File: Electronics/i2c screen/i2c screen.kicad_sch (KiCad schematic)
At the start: 4 parts, among them J1 renc_con, J2 display_con, J3 display_in, SW1 RotaryEncoder_Switch

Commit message: placement!
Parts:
- J1, J2, J3: footprint (none) -> Connector_PinHeader_2.54mm:PinHeader_1x04_P2.54mm_Vertical
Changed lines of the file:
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@@
 			)
 		)
-		(property "Footprint" ""
+		(property "Footprint" "Connector_PinHeader_2.54mm:PinHeader_1x04_P2.54mm_Vertical"
 			(at 101.6 76.2 0)
 			(effects
@@
 			)
 		)
-		(property "Footprint" ""
+		(property "Footprint" "Connector_PinHeader_2.54mm:PinHeader_1x04_P2.54mm_Vertical"
 			(at 123.19 60.96 0)
 			(effects
@@
 			)
 		)
-		(property "Footprint" ""
+		(property "Footprint" "Connector_PinHeader_2.54mm:PinHeader_1x04_P2.54mm_Vertical"
 			(at 116.84 76.2 0)
 			(effects

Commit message: updated footprints
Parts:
- J3: footprint Connector_PinHeader_2.54mm:PinHeader_1x04_P2.54mm_Vertical -> ledscreen:128x64OLED
- SW1: footprint (none) -> Rotary_Encoder:RotaryEncoder_Bourns_Vertical_PEC12R-3x17F-Sxxxx
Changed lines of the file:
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@@
 			)
 		)
-		(property "Footprint" ""
+		(property "Footprint" "Rotary_Encoder:RotaryEncoder_Bourns_Vertical_PEC12R-3x17F-Sxxxx"
 			(at 158.75 56.896 0)
 			(effects
@@
 			)
 		)
-		(property "Footprint" "Connector_PinHeader_2.54mm:PinHeader_1x04_P2.54mm_Vertical"
+		(property "Footprint" "ledscreen:128x64OLED"
 			(at 116.84 76.2 0)
 			(effects

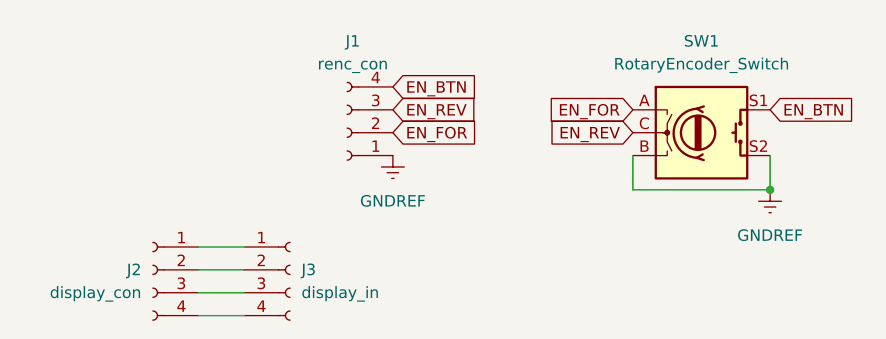
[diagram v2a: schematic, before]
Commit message: routing finito and placemnt aswell
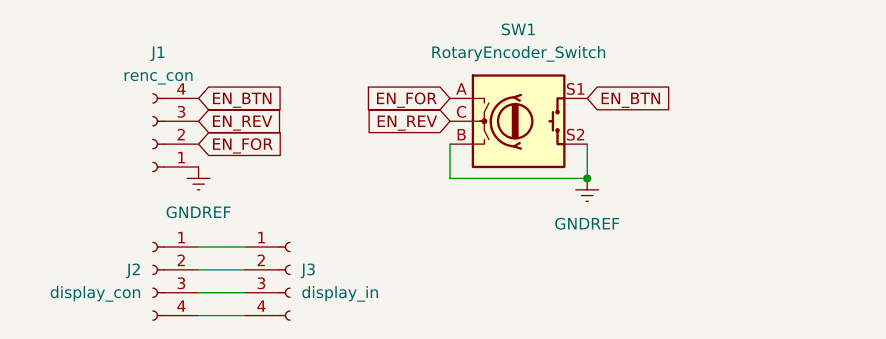
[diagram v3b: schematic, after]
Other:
- moved on the sheet: J1, SW1
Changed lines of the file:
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@@
 	(paper "A4")
 	(junction
-		(at 170.18 67.31)
+		(at 149.86 66.04)
 		(diameter 0)
 		(color 0 0 0 0)
@@
 	(wire
 		(pts
-			(xy 170.18 67.31) (xy 170.18 63.5)
+			(xy 149.86 66.04) (xy 149.86 62.23)
 		)
 		(stroke
@@
 	(wire
 		(pts
-			(xy 154.94 63.5) (xy 154.94 67.31)
+			(xy 134.62 62.23) (xy 134.62 66.04)
 		)
 		(stroke
@@
 	(wire
 		(pts
-			(xy 154.94 67.31) (xy 170.18 67.31)
+			(xy 134.62 66.04) (xy 149.86 66.04)
 		)
 		(stroke
@@
 	(global_label "EN_REV"
 		(shape input)
-		(at 154.94 60.96 180)
+		(at 134.62 59.69 180)
 		(fields_autoplaced yes)
 		(effects
@@
 		)
 		(property "Intersheetrefs" "${INTERSHEET_REFS}"
-			(at 145.0001 60.96 0)
+			(at 124.6801 59.69 0)
 			(effects
 				(font
@@
 	(global_label "EN_REV"
 		(shape input)
-		(at 128.27 58.42 0)
+		(at 106.68 59.69 0)
 		(fields_autoplaced yes)
 		(effects
@@
 		)
 		(property "Intersheetrefs" "${INTERSHEET_REFS}"
-			(at 138.2099 58.42 0)
+			(at 116.6199 59.69 0)
 			(effects
 				(font
@@
 	(global_label "EN_BTN"
 		(shape input)
-		(at 170.18 58.42 0)
+		(at 149.86 57.15 0)
 		(fields_autoplaced yes)
 		(effects
@@
 		)
 		(property "Intersheetrefs" "${INTERSHEET_REFS}"
-			(at 180.1804 58.42 0)
+			(at 159.8604 57.15 0)
 			(effects
 				(font
@@
 	(global_label "EN_FOR"
 		(shape input)
-		(at 128.27 60.96 0)
+		(at 106.68 62.23 0)
 		(fields_autoplaced yes)
 		(effects
@@
 		)
 		(property "Intersheetrefs" "${INTERSHEET_REFS}"
-			(at 138.3914 60.96 0)
+			(at 116.8014 62.23 0)
 			(effects
 				(font
@@
 	(global_label "EN_FOR"
 		(shape input)
-		(at 154.94 58.42 180)
+		(at 134.62 57.15 180)
 		(fields_autoplaced yes)
 		(effects
@@
 		)
 		(property "Intersheetrefs" "${INTERSHEET_REFS}"
-			(at 144.8186 58.42 0)
+			(at 124.4986 57.15 0)
 			(effects
 				(font
@@
 	(global_label "EN_BTN"
 		(shape input)
-		(at 128.27 55.88 0)
+		(at 106.68 57.15 0)
 		(fields_autoplaced yes)
 		(effects
@@
 		)
 		(property "Intersheetrefs" "${INTERSHEET_REFS}"
-			(at 138.2704 55.88 0)
+			(at 116.6804 57.15 0)
 			(effects
 				(font
@@
 	(symbol
 		(lib_id "Connector:Conn_01x04_Socket")
-		(at 123.19 60.96 180)
+		(at 101.6 62.23 180)
 		(unit 1)
 		(exclude_from_sim no)
@@
 		(fields_autoplaced yes)
 		(property "Reference" "J1"
-			(at 123.825 50.8 0)
+			(at 102.235 52.07 0)
 			(effects
 				(font
@@
 		)
 		(property "Value" "renc_con"
-			(at 123.825 53.34 0)
+			(at 102.235 54.61 0)
 			(effects
 				(font
@@
 		)
 		(property "Footprint" "Connector_PinHeader_2.54mm:PinHeader_1x04_P2.54mm_Vertical"
-			(at 123.19 60.96 0)
+			(at 101.6 62.23 0)
 			(effects
 				(font
@@
 		)
 		(property "Datasheet" "~"
-			(at 123.19 60.96 0)
+			(at 101.6 62.23 0)
 			(effects
 				(font
@@
 		)
 		(property "Description" "Generic connector, single row, 01x04, script generated"
-			(at 123.19 60.96 0)
+			(at 101.6 62.23 0)
 			(effects
 				(font
@@
 	(symbol
 		(lib_id "power:GNDREF")
-		(at 170.18 67.31 0)
+		(at 149.86 66.04 0)
 		(mirror y)
 		(unit 1)
@@
 		(fields_autoplaced yes)
 		(property "Reference" "#PWR02"
-			(at 170.18 73.66 0)
+			(at 149.86 72.39 0)
 			(effects
 				(font
@@
 		)
 		(property "Value" "GNDREF"
-			(at 170.18 72.39 0)
+			(at 149.86 71.12 0)
 			(effects
 				(font
@@
 		)
 		(property "Footprint" ""
-			(at 170.18 67.31 0)
+			(at 149.86 66.04 0)
 			(effects
 				(font
@@
 		)
 		(property "Datasheet" ""
-			(at 170.18 67.31 0)
+			(at 149.86 66.04 0)
 			(effects
 				(font
@@
 		)
 		(property "Description" ""
-			(at 170.18 67.31 0)
+			(at 149.86 66.04 0)
 			(effects
 				(font
@@
 	(symbol
 		(lib_id "power:GNDREF")
-		(at 128.27 63.5 0)
+		(at 106.68 64.77 0)
 		(mirror y)
 		(unit 1)
@@
 		(fields_autoplaced yes)
 		(property "Reference" "#PWR01"
-			(at 128.27 69.85 0)
+			(at 106.68 71.12 0)
 			(effects
 				(font
@@
 		)
 		(property "Value" "GNDREF"
-			(at 128.27 68.58 0)
+			(at 106.68 69.85 0)
 			(effects
 				(font
@@
 		)
 		(property "Footprint" ""
-			(at 128.27 63.5 0)
+			(at 106.68 64.77 0)
 			(effects
 				(font
@@
 		)
 		(property "Datasheet" ""
-			(at 128.27 63.5 0)
+			(at 106.68 64.77 0)
 			(effects
 				(font
@@
 		)
 		(property "Description" ""
-			(at 128.27 63.5 0)
+			(at 106.68 64.77 0)
 			(effects
 				(font
@@
 	(symbol
 		(lib_id "Device:RotaryEncoder_Switch")
-		(at 162.56 60.96 0)
+		(at 142.24 59.69 0)
 		(unit 1)
 		(exclude_from_sim no)
@@
 		(dnp no)
 		(property "Reference" "SW1"
-			(at 162.56 50.8 0)
+			(at 142.24 49.53 0)
 			(effects
 				(font
@@
 		)
 		(property "Value" "RotaryEncoder_Switch"
-			(at 162.56 53.34 0)
+			(at 142.24 52.07 0)
 			(effects
 				(font
@@
 		)
 		(property "Footprint" "Rotary_Encoder:RotaryEncoder_Bourns_Vertical_PEC12R-3x17F-Sxxxx"
-			(at 158.75 56.896 0)
+			(at 138.43 55.626 0)
 			(effects
 				(font
@@
 		)
 		(property "Datasheet" "~"
-			(at 162.56 54.356 0)
+			(at 142.24 53.086 0)
 			(effects
 				(font
@@
 		)
 		(property "Description" "Rotary encoder, dual channel, incremental quadrate outputs, with switch"
-			(at 162.56 60.96 0)
-			(effects
-				(font
+			(at 142.24 59.69 0)
+			(effects
+				(font
